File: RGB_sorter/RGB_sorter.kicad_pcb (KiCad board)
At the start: 4 copper layers, 70 x 100.5 mm, 51 parts, among them J1 Servo, J10 TCS34725, J11 IR sensor, J2 Power, J3 Motor A, J4 Motor B, J6 LCD, J8 Conn_01x05_Pin, SW1 START, SW2 RESET, SW3 STOP, U1 L298N, U2 L7805, U3 ULN2003, U4 NUCLEO64-F411RE

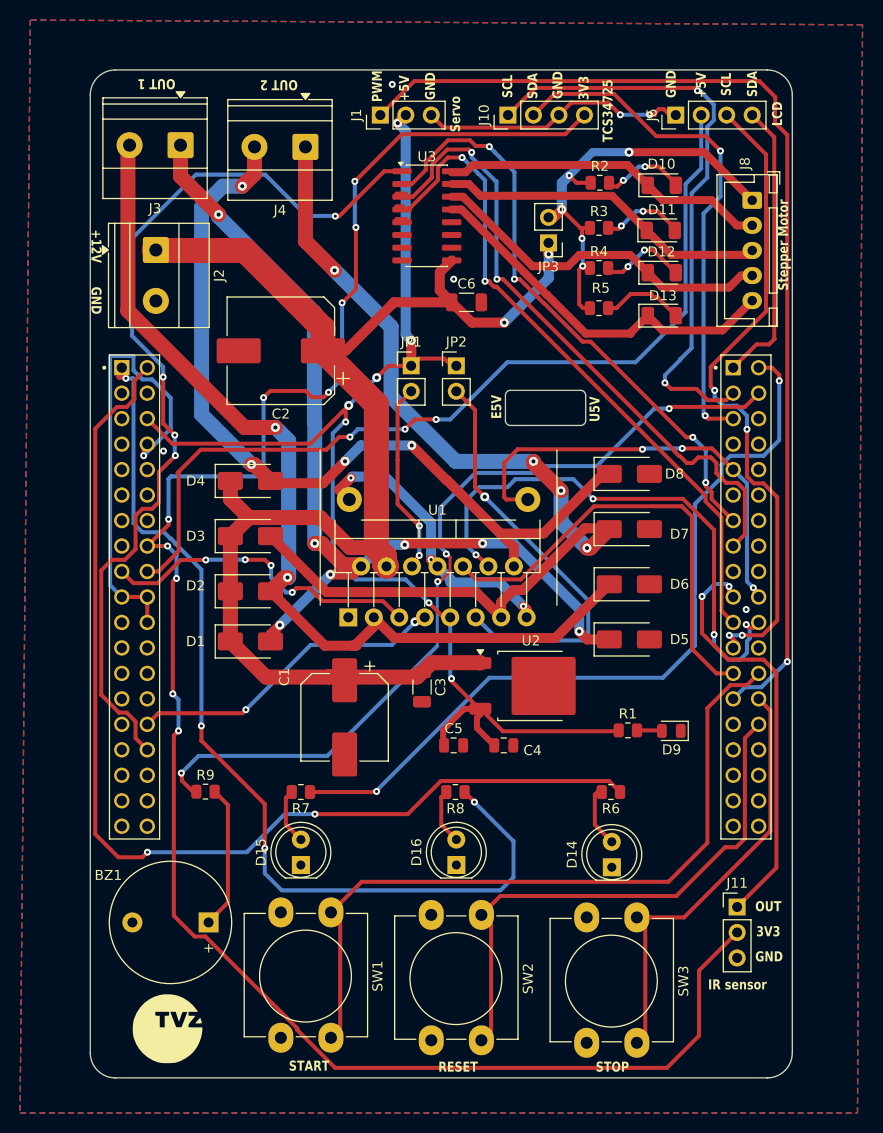
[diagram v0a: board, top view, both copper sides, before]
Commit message: Upgrade PCB-a
Shematic i PCB edit
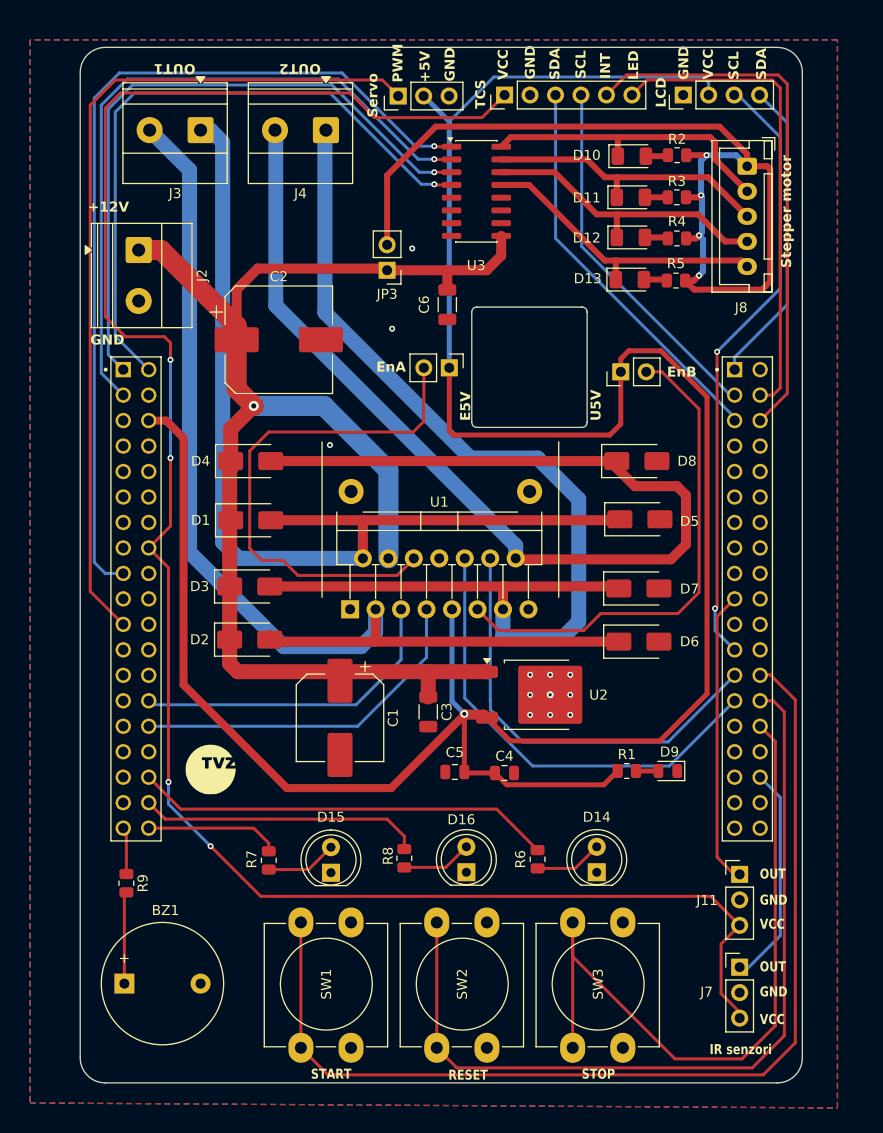
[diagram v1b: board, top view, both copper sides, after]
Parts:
- removed J10: TCS34725, Connector_PinHeader_2.54mm:PinHeader_1x04_P2.54mm_Vertical
- added J5: TCS34725, Connector_PinHeader_2.54mm:PinHeader_1x06_P2.54mm_Vertical, F.Cu at (122.8, 34.5)
- added J7: IR sensor2, Connector_PinHeader_2.54mm:PinHeader_1x03_P2.54mm_Vertical, F.Cu at (146.2, 121.5)
- D16: value LED_Blue -> LED_Orange
- J11: value IR sensor -> IR sensor1
- moved G*** 26.2 mm to (93.5, 101.8)
- moved JP2 16.4 mm to (134.4, 62.1), turned to 90 degrees
- moved JP3 16.3 mm to (111.1, 52.0)
- moved SW3 14.5 mm to (129.6, 129.5), turned to 90 degrees
- moved SW2 14.0 mm to (116.0, 129.5), turned to 90 degrees
- moved SW1 13.8 mm to (102.5, 129.5), turned to 90 degrees
- moved D1 12.1 mm to (97.5, 76.9)
- moved R9 12.1 mm to (85.1, 113.1), turned to -90 degrees
- moved D5 12.0 mm to (136.3, 76.8)
- moved BZ1 10.4 mm to (84.9, 123.1), turned to 0 degrees
- moved R6 9.92 mm to (126.1, 110.7), turned to -90 degrees
- moved R8 8.34 mm to (112.8, 110.6), turned to -90 degrees
- moved R3 8.34 mm to (140.0, 44.7), turned to 180 degrees
- moved R4 8.32 mm to (140.0, 48.8), turned to 180 degrees
- moved R2 8.18 mm to (140.0, 40.5), turned to 180 degrees
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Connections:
- net IN2 renamed /IN2
- net Net-(J11-Pin_1) renamed /IR_OUT
- net Net-(SW1-A) renamed /START
- net PA8 renamed /LCD_SCL
- net PC9 renamed /LCD_SDA
- J1 pad 1: PB4 -> /SERVO_PWM
- J11 pad 2: +3V3 -> GND
- J11 pad 3: GND -> +3.3V
- J6 pad 2: Net-(J6-Pin_2) -> +5V
- R6 pad 1: Net-(U4-PC11) -> /RED
- R7 pad 1: Net-(U4-PC8) -> /GREEN
- R8 pad 1: Net-(U4-PC10) -> /ORANGE
- R9 pad 1: Net-(U4-PC6) -> /BUZZER
- SW2 pad 1: Net-(SW2-A) -> /RESET
- SW3 pad 1: Net-(SW3-A) -> /STOP
- U1 pad 10: IN3 -> /IN3
- U1 pad 12: IN4 -> /IN4
- U1 pad 5: IN1 -> /IN1
- U3 pad 1: I1 -> /I1
- U3 pad 2: I2 -> /I2
- U3 pad 3: I3 -> /I3
- U3 pad 4: I4 -> /I4
- U4 pad 1: Net-(U4-PC10) -> /I3
- U4 pad 16: +3V3 -> +3.3V
- U4 pad 17: IN1 -> /I1
- U4 pad 18: Net-(J6-Pin_2) -> unconnected-(U4-+5V-Pad18)
- U4 pad 2: Net-(U4-PC11) -> /I4
- U4 pad 21: unconnected-(U4-PB7-Pad21) -> /SERVO_PWM
- U4 pad 28: unconnected-(U4-PA0-Pad28) -> /IN1
- U4 pad 3: unconnected-(U4-PC12-Pad3) -> /I2
- U4 pad 32: I1 -> unconnected-(U4-PA4-Pad32)
- U4 pad 34: unconnected-(U4-PB0-Pad34) -> /RED
- U4 pad 36: unconnected-(U4-PC1-Pad36) -> /ORANGE
- U4 pad 37: unconnected-(U4-PC3-Pad37) -> /BUZZER
- U4 pad 38: unconnected-(U4-PC0-Pad38) -> /GREEN
- U4 pad 40: Net-(U4-PC8) -> unconnected-(U4-PC8-Pad40)
- U4 pad 41: Net-(J10-Pin_1) -> /TCS_SCL
- U4 pad 42: Net-(U4-PC6) -> /LED
- U4 pad 43: Net-(J10-Pin_2) -> /TCS_SDA
- U4 pad 44: unconnected-(U4-PC5-Pad44) -> /INT
- U4 pad 51: I2 -> unconnected-(U4-PA6-Pad51)
- U4 pad 53: I3 -> unconnected-(U4-PA7-Pad53)
- U4 pad 59: I4 -> unconnected-(U4-PA9-Pad59)
- U4 pad 60: IN4 -> unconnected-(U4-PB2-Pad60)
- U4 pad 63: IN3 -> /IN4
- U4 pad 65: PB4 -> /IN3
- U4 pad 66: Net-(SW3-A) -> /RESET
- U4 pad 68: Net-(SW2-A) -> /STOP
- U4 pad 72: unconnected-(U4-PC4-Pad72) -> /IR2_OUT
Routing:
- net +3V3: track 191.8 -> 0.00 mm, vias 10 -> 0
- net +3.3V: track 0.00 -> 191.7 mm, vias 0 -> 4
- net GND: track 146.6 -> 0.42 mm, vias 13 -> 12
- net +5V: track 127.1 -> 253.0 mm, vias 7 -> 1
- net Net-(U4-PC11): track 106.1 -> 0.00 mm, vias 2 -> 0
- net PB4: track 105.2 -> 0.00 mm, vias 1 -> 0
- net Net-(U4-PC10): track 96.0 -> 0.00 mm, vias 4 -> 0
- net I1: track 92.6 -> 0.00 mm, vias 4 -> 0
- net Net-(J6-Pin_2): track 89.4 -> 0.00 mm, vias 3 -> 0
- net /I1: track 0.00 -> 89.4 mm, vias 0 -> 1
- net /RESET: track 0.00 -> 86.0 mm
- net /SERVO_PWM: track 0.00 -> 85.4 mm
- net Net-(U4-PC6): track 84.9 -> 0.00 mm, vias 4 -> 0
- net Net-(U4-PC8): track 79.3 -> 0.00 mm, vias 2 -> 0
- net /STOP: track 0.00 -> 72.2 mm
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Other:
- board size 70 x 100.5 mm -> 72 x 103.2 mm
- copper layers 4 -> 2
- board text added: "EnA"
- board text added: "EnB"
- board text added: "INT"
- board text added: "IR senzori"
- board text added: "LED"
- board text added: "OUT1"
- board text added: "OUT2"
- board text added: "Stepper motor"
- board text added: "TCS"
- board text added: "VCC"
- board text removed: "3V3"
- board text removed: "IR sensor"
- board text removed: "OUT 1"
- board text removed: "OUT 2"
- board text removed: "Stepper Motor"
- board text removed: "TCS34725"
